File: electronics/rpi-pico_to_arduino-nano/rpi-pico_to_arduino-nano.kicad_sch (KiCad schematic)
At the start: 2 parts, among them U1 Pico

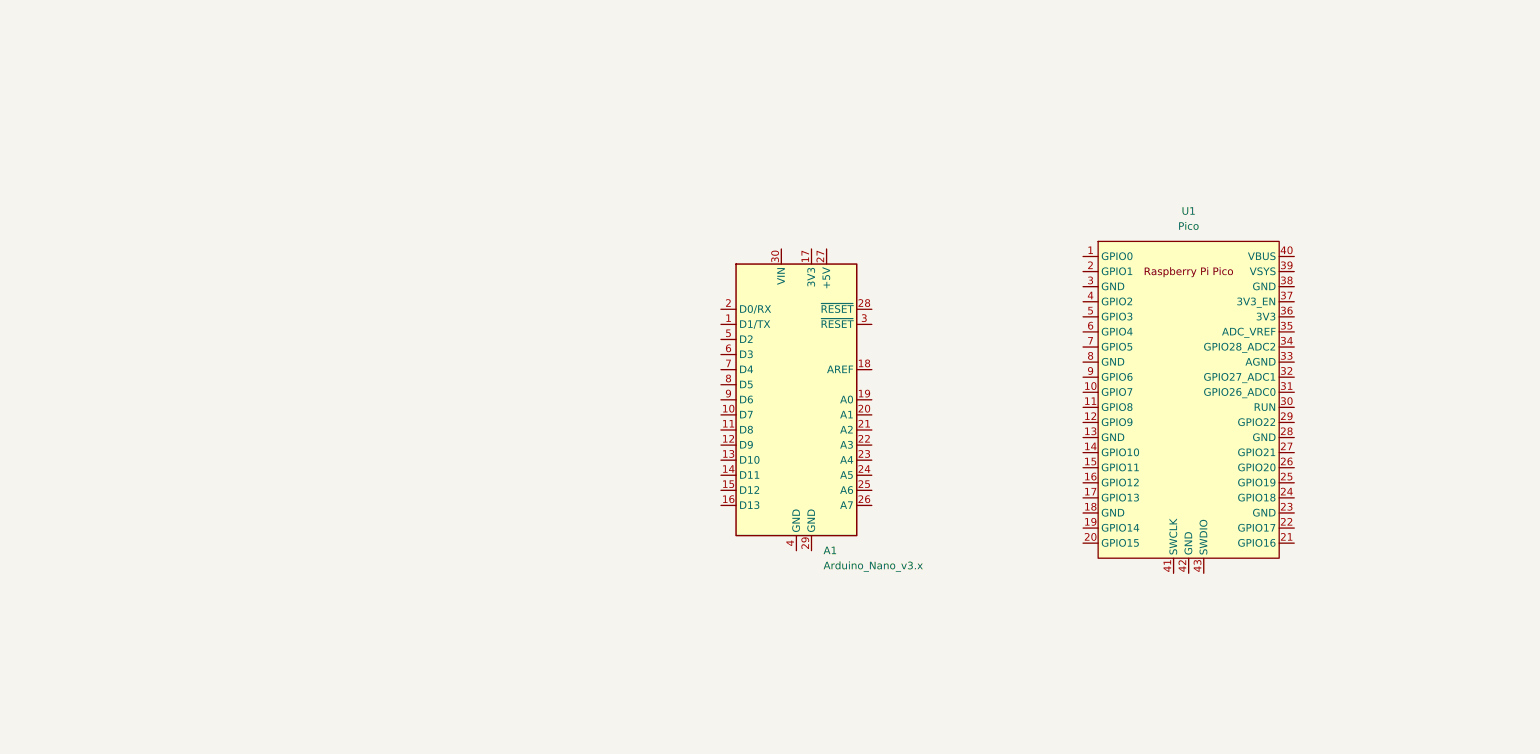
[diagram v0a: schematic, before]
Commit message: add some connections and comments
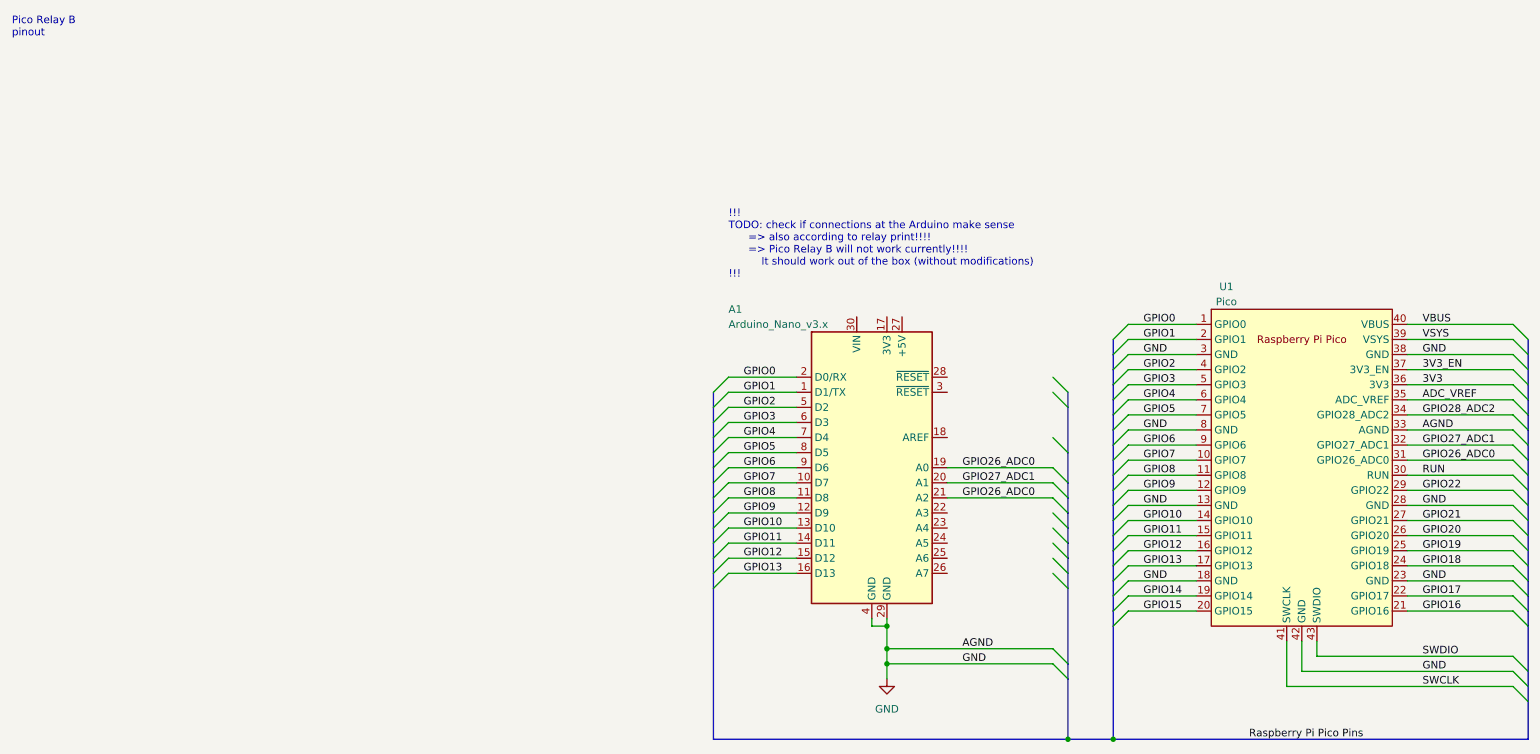
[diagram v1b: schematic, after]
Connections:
- net GPIO0: now reaches U1.1 (GPIO0)
- net GPIO0: now also A1.2 (D0/RX)
- net GPIO7: now reaches U1.10 (GPIO7)
- net GPIO7: now also A1.10 (D7)
- net GPIO8: now reaches U1.11 (GPIO8)
- net GPIO8: now also A1.11 (D8)
- net GPIO9: now reaches U1.12 (GPIO9)
- net GPIO9: now also A1.12 (D9)
- net GND: now reaches U1.13 (GND)
- net GND: now also A1.29 (GND), A1.4 (GND), U1.18 (GND), U1.23 (GND), U1.28 (GND), U1.3 (GND), U1.33 (AGND), U1.38 (GND), U1.42 (GND), U1.8 (GND)
- net GPIO10: now reaches U1.14 (GPIO10)
- net GPIO10: now also A1.13 (D10)
- net GPIO11: now reaches U1.15 (GPIO11)
- net GPIO11: now also A1.14 (D11)
- net GPIO12: now reaches U1.16 (GPIO12)
- net GPIO12: now also A1.15 (D12)
- net GPIO13: now reaches U1.17 (GPIO13)
- net GPIO13: now also A1.16 (D13)
- net GPIO14: now reaches U1.19 (GPIO14)
- net GPIO1: now reaches U1.2 (GPIO1)
- net GPIO1: now also A1.1 (D1/TX)
- net GPIO15: now reaches U1.20 (GPIO15)
- net GPIO16: now reaches U1.21 (GPIO16)
- net GPIO17: now reaches U1.22 (GPIO17)
- net GPIO18: now reaches U1.24 (GPIO18)
- net GPIO19: now reaches U1.25 (GPIO19)
- net GPIO20: now reaches U1.26 (GPIO20)
- net GPIO21: now reaches U1.27 (GPIO21)
- net GPIO22: now reaches U1.29 (GPIO22)
- net RUN: now reaches U1.30 (RUN)
- net GPIO26_ADC0: now reaches U1.31 (GPIO26_ADC0)
- net GPIO26_ADC0: now also A1.19 (A0), A1.21 (A2)
- net GPIO27_ADC1: now reaches U1.32 (GPIO27_ADC1)
- net GPIO27_ADC1: now also A1.20 (A1)
- net GPIO28_ADC2: now reaches U1.34 (GPIO28_ADC2)
- net ADC_VREF: now reaches U1.35 (ADC_VREF)
- net 3V3: now reaches U1.36 (3V3)
- net 3V3_EN: now reaches U1.37 (3V3_EN)
- net VSYS: now reaches U1.39 (VSYS)
- net GPIO2: now reaches U1.4 (GPIO2)
- net GPIO2: now also A1.5 (D2)
- net VBUS: now reaches U1.40 (VBUS)
- net SWCLK: now reaches U1.41 (SWCLK)
- net SWDIO: now reaches U1.43 (SWDIO)
- net GPIO3: now reaches U1.5 (GPIO3)
- net GPIO3: now also A1.6 (D3)
- net GPIO4: now reaches U1.6 (GPIO4)
- net GPIO4: now also A1.7 (D4)
- net GPIO5: now reaches U1.7 (GPIO5)
- net GPIO5: now also A1.8 (D5)
- net GPIO6: now reaches U1.9 (GPIO6)
- net GPIO6: now also A1.9 (D6)
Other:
- note added: "!!! TODO: check if connections at the Arduino make sense => also according to relay print!!!! => Pico Relay B will not work currently!!!! It should work out of the box (without modifications) !!!"
- note added: "Pico Relay B pinout"
- moved on the sheet: A1, U1
